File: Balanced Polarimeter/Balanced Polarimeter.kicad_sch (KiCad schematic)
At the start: 23 parts, among them IC1 OP27, J1 73100-0105, J2 Conn_01x03_Pin, J3 Conn_01x02_Pin, J5 Conn_01x02_Pin, Q1 MMPQ3904, Q2 MMPQ3904, U1 ADA4898-1YRDZ, U2 ADA4898-1YRDZ

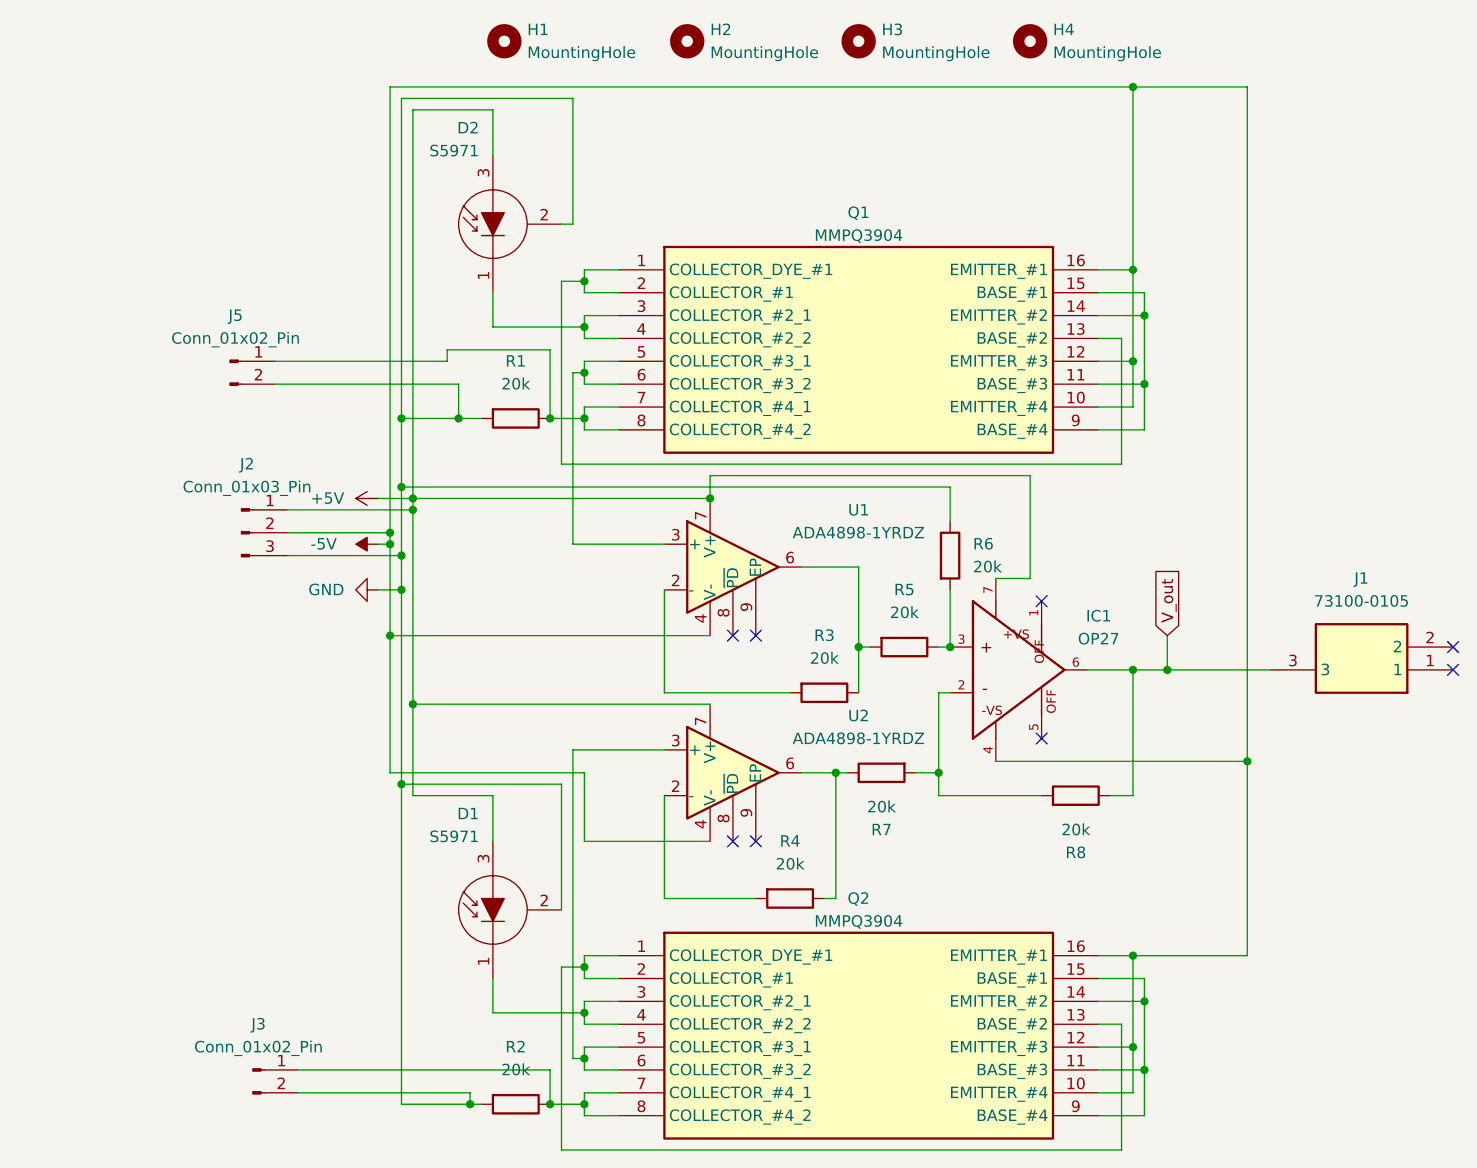
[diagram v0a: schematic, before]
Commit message: Revised Wiring
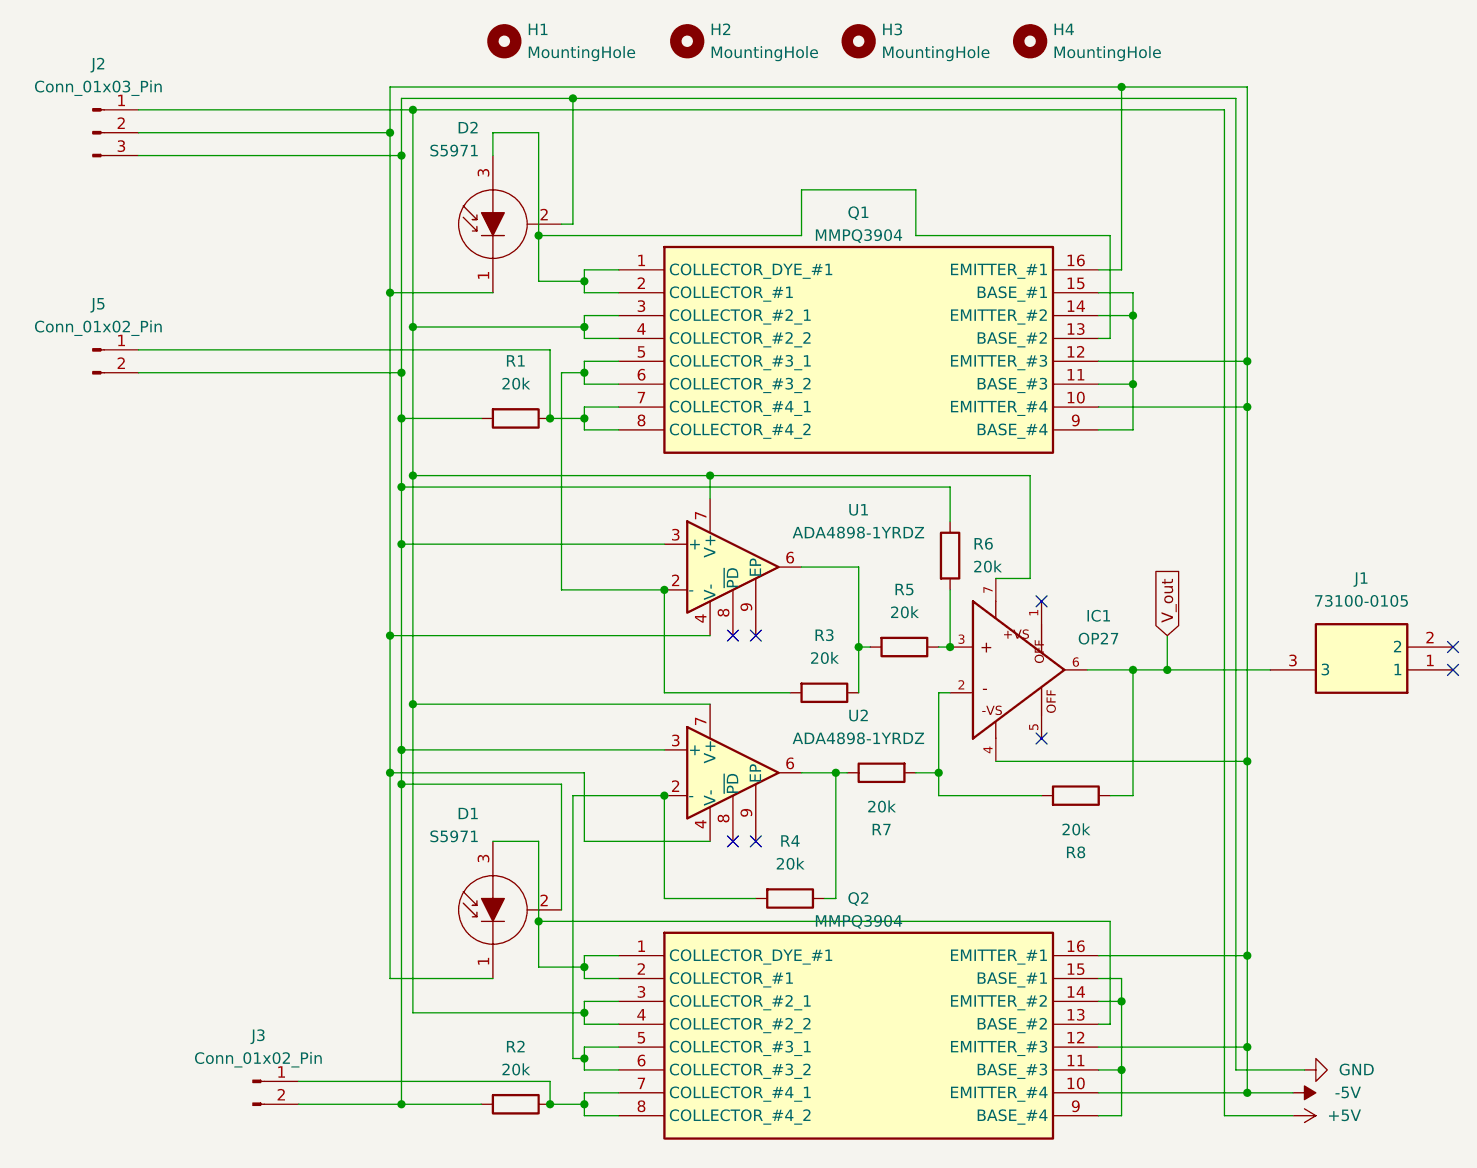
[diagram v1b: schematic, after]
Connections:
- net +5V: now also Q1.3 (COLLECTOR_#2_1), Q1.4 (COLLECTOR_#2_2), Q2.3 (COLLECTOR_#2_1), Q2.4 (COLLECTOR_#2_2); no longer D1.3 (A), D2.3 (A)
- net -5V: now also D1.1 (K), D2.1 (K)
- net GND: now also U1.3 (+), U2.3 (+)
- net at Q2.1 (COLLECTOR_DYE_#1), Q2.13 (BASE_#2), Q2.2 (COLLECTOR_#1): now also D1.3 (A)
- net at Q2.5 (COLLECTOR_#3_1), Q2.6 (COLLECTOR_#3_2): now also R4.2, U2.2 (-); no longer U2.3 (+)
- net at Q1.1 (COLLECTOR_DYE_#1), Q1.13 (BASE_#2), Q1.2 (COLLECTOR_#1): now also D2.3 (A)
- net at Q1.5 (COLLECTOR_#3_1), Q1.6 (COLLECTOR_#3_2): now also R3.2, U1.2 (-); no longer U1.3 (+)
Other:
- moved on the sheet: J2, J3, J5
